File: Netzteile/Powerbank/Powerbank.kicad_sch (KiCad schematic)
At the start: 40 parts, among them J1 Conn_01x04_Female, J2 Conn_01x06_Female

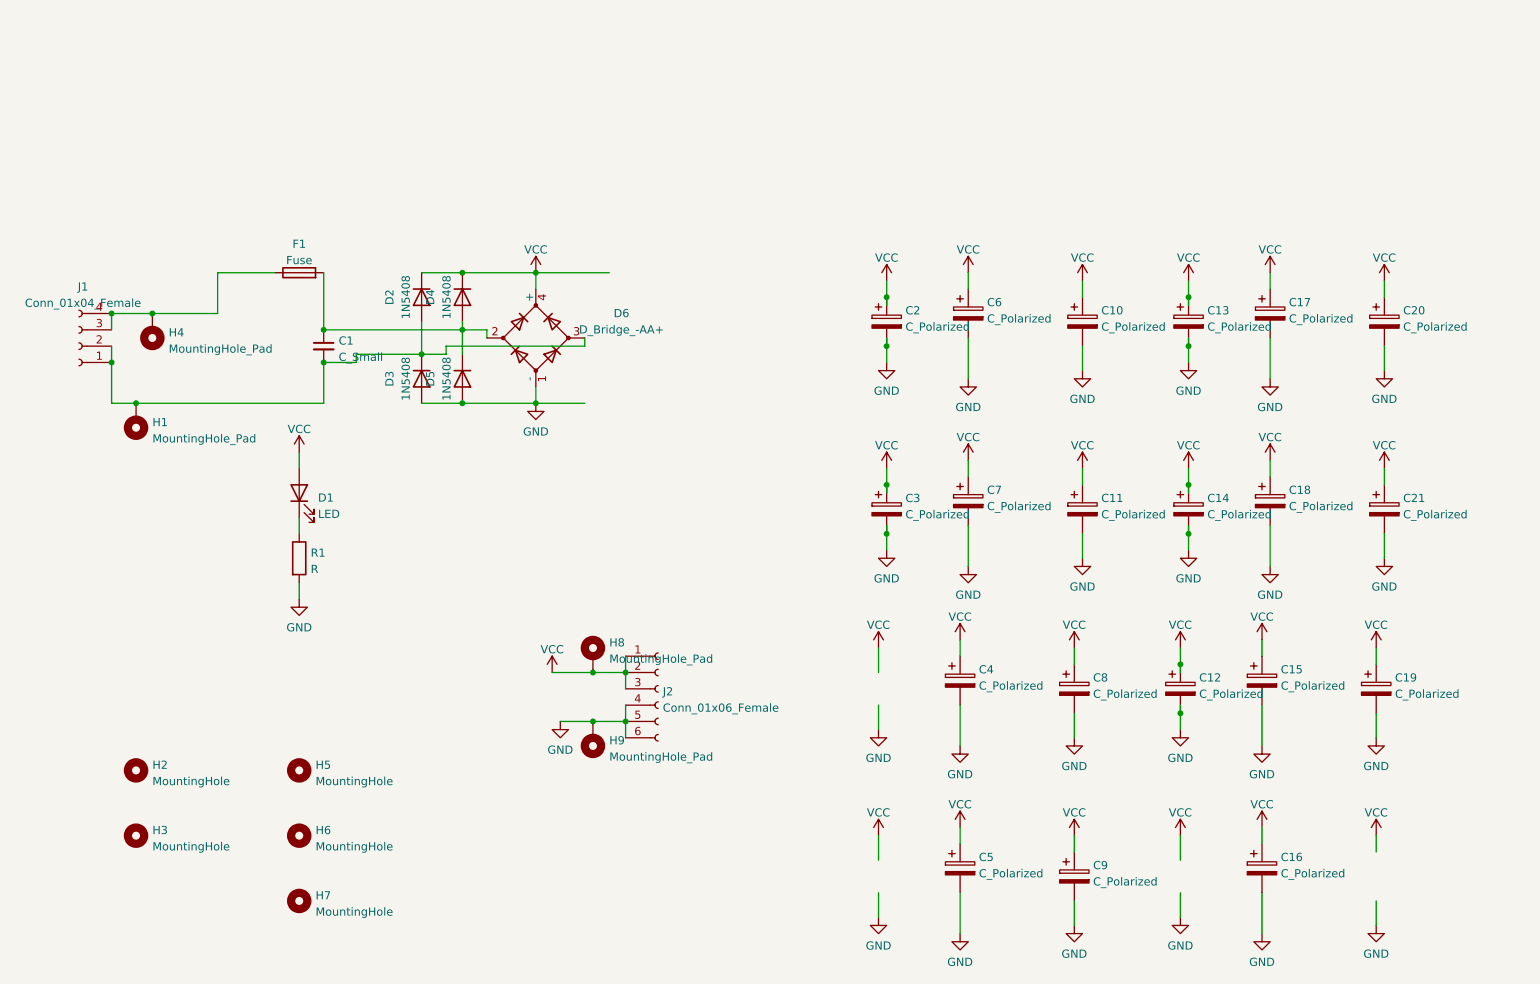
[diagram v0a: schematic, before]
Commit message: Umsortiert
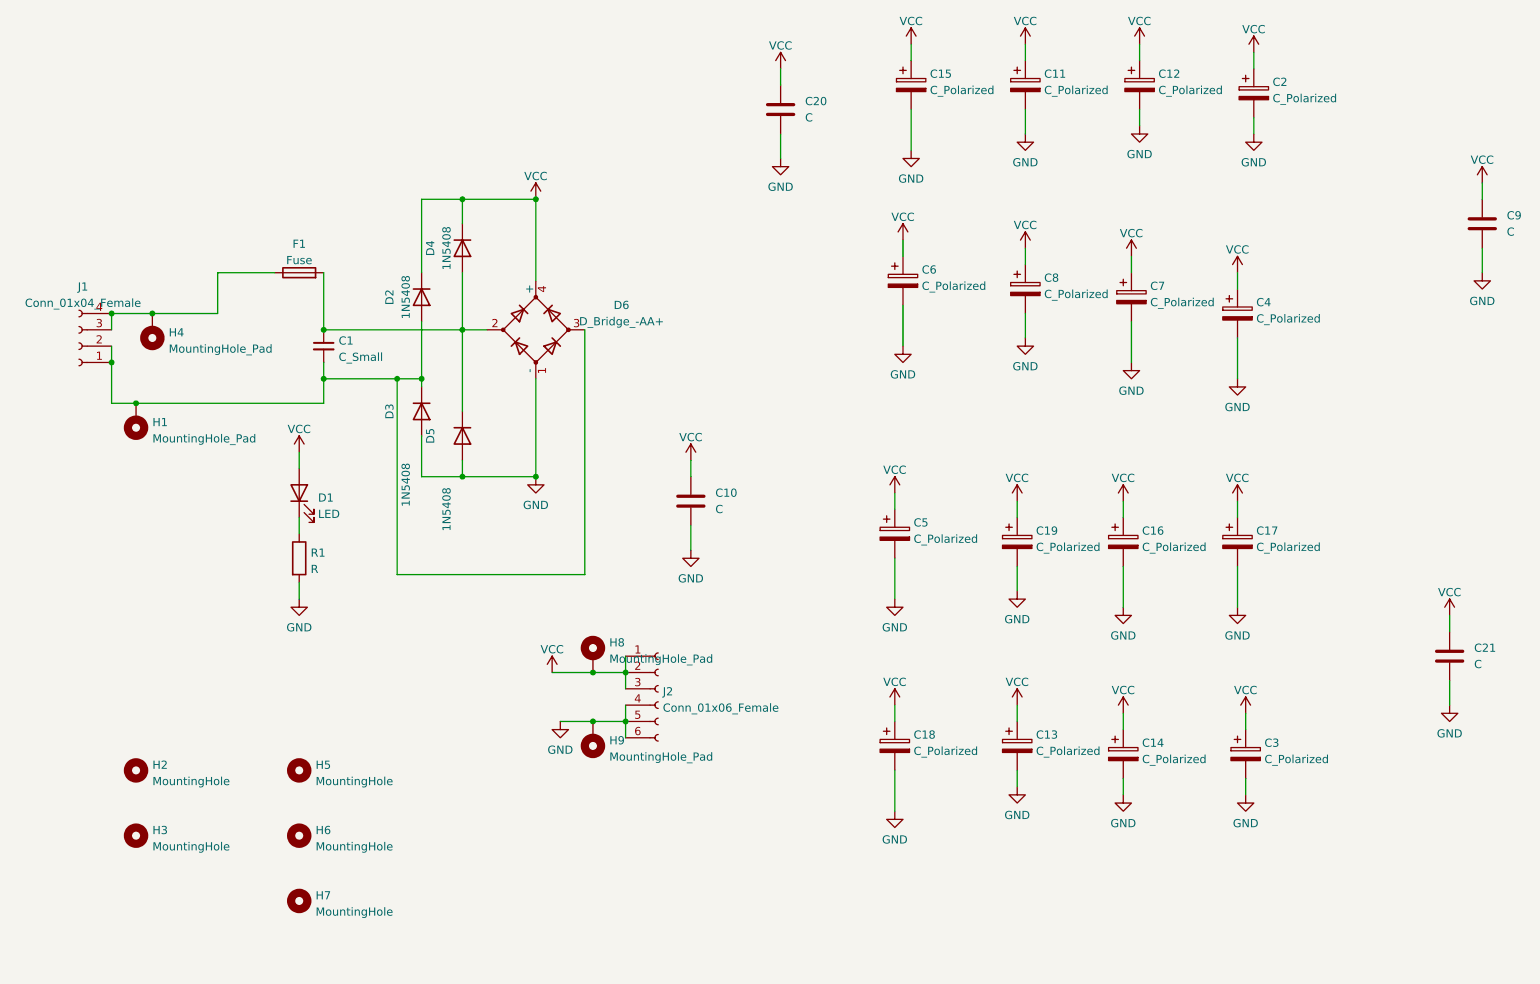
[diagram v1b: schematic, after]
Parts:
- removed C10, C20, C21, C9: C_Polarized, Capacitor_THT:C_Rect_L16.5mm_W5.0mm_P15.00mm_MKT, symbol Device:C_Polarized
- added C10, C20, C21, C9: C, Capacitor_THT:C_Rect_L16.5mm_W5.0mm_P15.00mm_MKT, symbol Device:C
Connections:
- net GND: now also C10.2, C20.2, C21.2, C9.2
- net VCC: now also C10.1, C20.1, C21.1, C9.1
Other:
- moved on the sheet: C11, C12, C13, C14, C15, C16, C17, C18, C19, C2, C3, C4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
